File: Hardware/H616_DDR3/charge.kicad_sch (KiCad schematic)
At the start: 21 parts, among them J4 USB_C_Receptacle_USB2.0, Q1 AO3420_C358680, SW1 CK_KMS2xxG, U4 SW6206, U5 BX-PH2_0-2PZZ

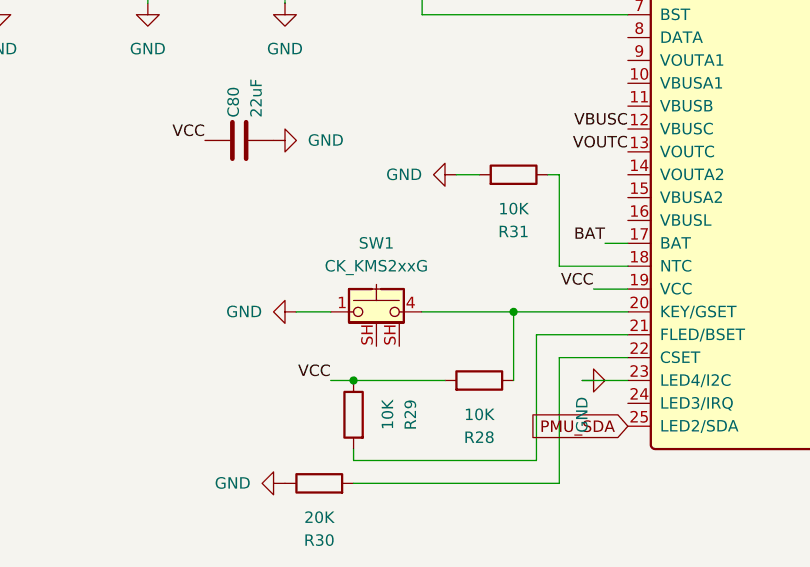
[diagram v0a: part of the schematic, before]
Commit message: Errors fix
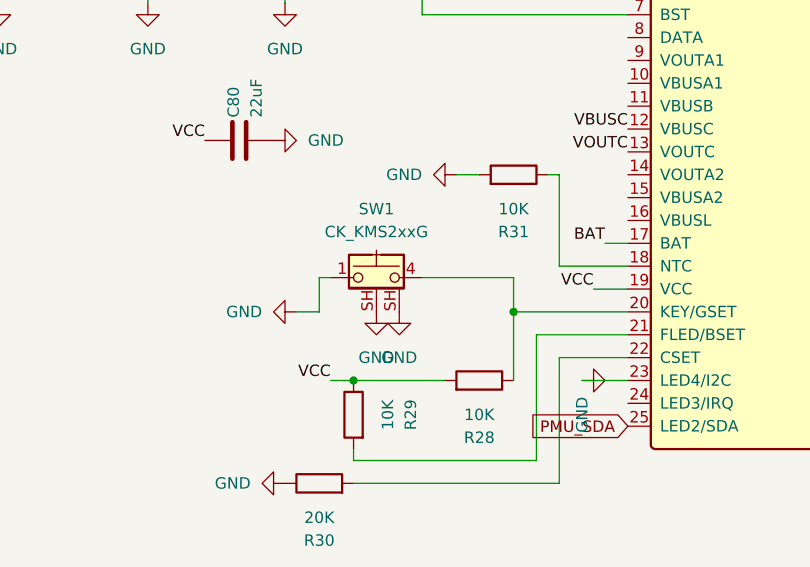
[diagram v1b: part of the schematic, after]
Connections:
- net GND: now also SW1.SH (3)
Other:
- moved on the sheet: SW1
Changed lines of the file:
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@@
 	(wire
 		(pts
+			(xy 67.31 93.98) (xy 67.31 97.79)
+		)
+		(stroke
+			(width 0)
+			(type default)
+		)
+	)
+	(wire
+		(pts
 			(xy 248.92 139.7) (xy 251.46 139.7)
 		)
@@
 	(wire
 		(pts
-			(xy 64.77 97.79) (xy 68.58 97.79)
+			(xy 67.31 93.98) (xy 68.58 93.98)
 		)
 		(stroke
@@
 	(wire
 		(pts
+			(xy 88.9 93.98) (xy 88.9 97.79)
+		)
+		(stroke
+			(width 0)
+			(type default)
+		)
+	)
+	(wire
+		(pts
 			(xy 248.92 137.16) (xy 251.46 137.16)
 		)
@@
 	(wire
 		(pts
-			(xy 78.74 97.79) (xy 88.9 97.79)
+			(xy 78.74 93.98) (xy 88.9 93.98)
 		)
 		(stroke
@@
 	(wire
 		(pts
+			(xy 67.31 97.79) (xy 64.77 97.79)
+		)
+		(stroke
+			(width 0)
+			(type default)
+		)
+	)
+	(wire
+		(pts
 			(xy 88.9 97.79) (xy 101.6 97.79)
 		)
@@
 	)
 	(symbol
+		(lib_id "power:GND")
+		(at 73.66 97.79 0)
+		(unit 1)
+		(body_style 1)
+		(exclude_from_sim no)
+		(in_bom yes)
+		(on_board yes)
+		(in_pos_files yes)
+		(dnp no)
+		(fields_autoplaced yes)
+		(property "Reference" "#PWR016"
+			(at 73.66 104.14 0)
+			(hide yes)
+			(show_name no)
+			(do_not_autoplace no)
+			(effects
+				(font
+					(size 1.27 1.27)
+				)
+			)
+		)
+		(property "Value" "GND"
+			(at 73.66 102.87 0)
+			(show_name no)
+			(do_not_autoplace no)
+			(effects
+				(font
+					(size 1.27 1.27)
+				)
+			)
+		)
+		(property "Footprint" ""
+			(at 73.66 97.79 0)
+			(hide yes)
+			(show_name no)
+			(do_not_autoplace no)
+			(effects
+				(font
+					(size 1.27 1.27)
+				)
+			)
+		)
+		(property "Datasheet" ""
+			(at 73.66 97.79 0)
+			(hide yes)
+			(show_name no)
+			(do_not_autoplace no)
+			(effects
+				(font
+					(size 1.27 1.27)
+				)
+			)
+		)
+		(property "Description" "Power symbol creates a global label with name \"GND\" , ground"
+			(at 73.66 97.79 0)
+			(hide yes)
+			(show_name no)
+			(do_not_autoplace no)
+			(effects
+				(font
+					(size 1.27 1.27)
+				)
+			)
+		)
+		(pin "1"
+		)
+		(instances
+			(project "H616_devboard"
+				(path "/44f68964-8d75-4db0-b784-705712e148bc/34c0604f-0eea-4ed0-a3f4-7af63e92cae5"
+					(reference "#PWR016")
+					(unit 1)
+				)
+			)
+		)
+	)
+	(symbol
 		(lib_id "Device:C")
 		(at 154.94 77.47 90)
@@
 	(symbol
 		(lib_id "power:GND")
+		(at 76.2 97.79 0)
+		(unit 1)
+		(body_style 1)
+		(exclude_from_sim no)
+		(in_bom yes)
+		(on_board yes)
+		(in_pos_files yes)
+		(dnp no)
+		(fields_autoplaced yes)
+		(property "Reference" "#PWR042"
+			(at 76.2 104.14 0)
+			(hide yes)
+			(show_name no)
+			(do_not_autoplace no)
+			(effects
+				(font
+					(size 1.27 1.27)
+				)
+			)
+		)
+		(property "Value" "GND"
+			(at 76.2 102.87 0)
+			(show_name no)
+			(do_not_autoplace no)
+			(effects
+				(font
+					(size 1.27 1.27)
+				)
+			)
+		)
+		(property "Footprint" ""
+			(at 76.2 97.79 0)
+			(hide yes)
+			(show_name no)
+			(do_not_autoplace no)
+			(effects
+				(font
+					(size 1.27 1.27)
+				)
+			)
+		)
+		(property "Datasheet" ""
+			(at 76.2 97.79 0)
+			(hide yes)
+			(show_name no)
+			(do_not_autoplace no)
+			(effects
+				(font
+					(size 1.27 1.27)
+				)
+			)
+		)
+		(property "Description" "Power symbol creates a global label with name \"GND\" , ground"
+			(at 76.2 97.79 0)
+			(hide yes)
+			(show_name no)
+			(do_not_autoplace no)
+			(effects
+				(font
+					(size 1.27 1.27)
+				)
+			)
+		)
+		(pin "1"
+		)
+		(instances
+			(project "H616_devboard"
+				(path "/44f68964-8d75-4db0-b784-705712e148bc/34c0604f-0eea-4ed0-a3f4-7af63e92cae5"
+					(reference "#PWR042")
+					(unit 1)
+				)
+			)
+		)
+	)
+	(symbol
+		(lib_id "power:GND")
 		(at 63.5 63.5 0)
 		(unit 1)
@@
 	(symbol
 		(lib_id "Switch:CK_KMS2xxG")
-		(at 73.66 97.79 0)
+		(at 73.66 93.98 0)
 		(unit 1)
 		(body_style 1)
@@
 		(fields_autoplaced yes)
 		(property "Reference" "SW1"
-			(at 73.66 90.17 0)
+			(at 73.66 86.36 0)
 			(show_name no)
 			(do_not_autoplace no)
@@
 		)
 		(property "Value" "CK_KMS2xxG"
-			(at 73.66 92.71 0)
+			(at 73.66 88.9 0)
 			(show_name no)
 			(do_not_autoplace no)
@@
 		)
 		(property "Footprint" "bodya:button 3x6x3.5mm"
-			(at 73.66 92.71 0)
+			(at 73.66 88.9 0)
 			(hide yes)
 			(show_name no)
@@
 		)
 		(property "Datasheet" "https://www.ckswitches.com/media/1482/kms.pdf"
-			(at 73.66 92.71 0)
+			(at 73.66 88.9 0)
 			(hide yes)
 			(show_name no)
@@
 		)
 		(property "Description" "Microminiature SMT Side Actuated, 4.2 x 2.8 x 1.42mm, without pegs, with shield pin"
-			(at 73.66 97.79 0)
+			(at 73.66 93.98 0)
 			(hide yes)
 			(show_name no)
